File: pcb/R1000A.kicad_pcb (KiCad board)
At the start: 2 copper layers, 162 x 104 mm, 26 parts, among them J1 PCIESOCKET-X1, J10 PCIESOCKET-X1, J11 PCIESOCKET-X1, J12 PCIESOCKET-X1, J13 PCIESOCKET-X1, J14 PCIESOCKET-X1, J15 SOCKET420P-02X04-CPU, J16 SOCKET508P-01X04, J17 CONN500P-01X04, J2 PCIESOCKET-X1, J3 PCIESOCKET-X1, J4 PCIESOCKET-X1, J5 PCIESOCKET-X1, J6 PCIESOCKET-X1, J7 PCIESOCKET-X1, J8 PCIESOCKET-X1, J9 PCIESOCKET-X1, U1 LPC1769FBD100,551, U2 AP3418

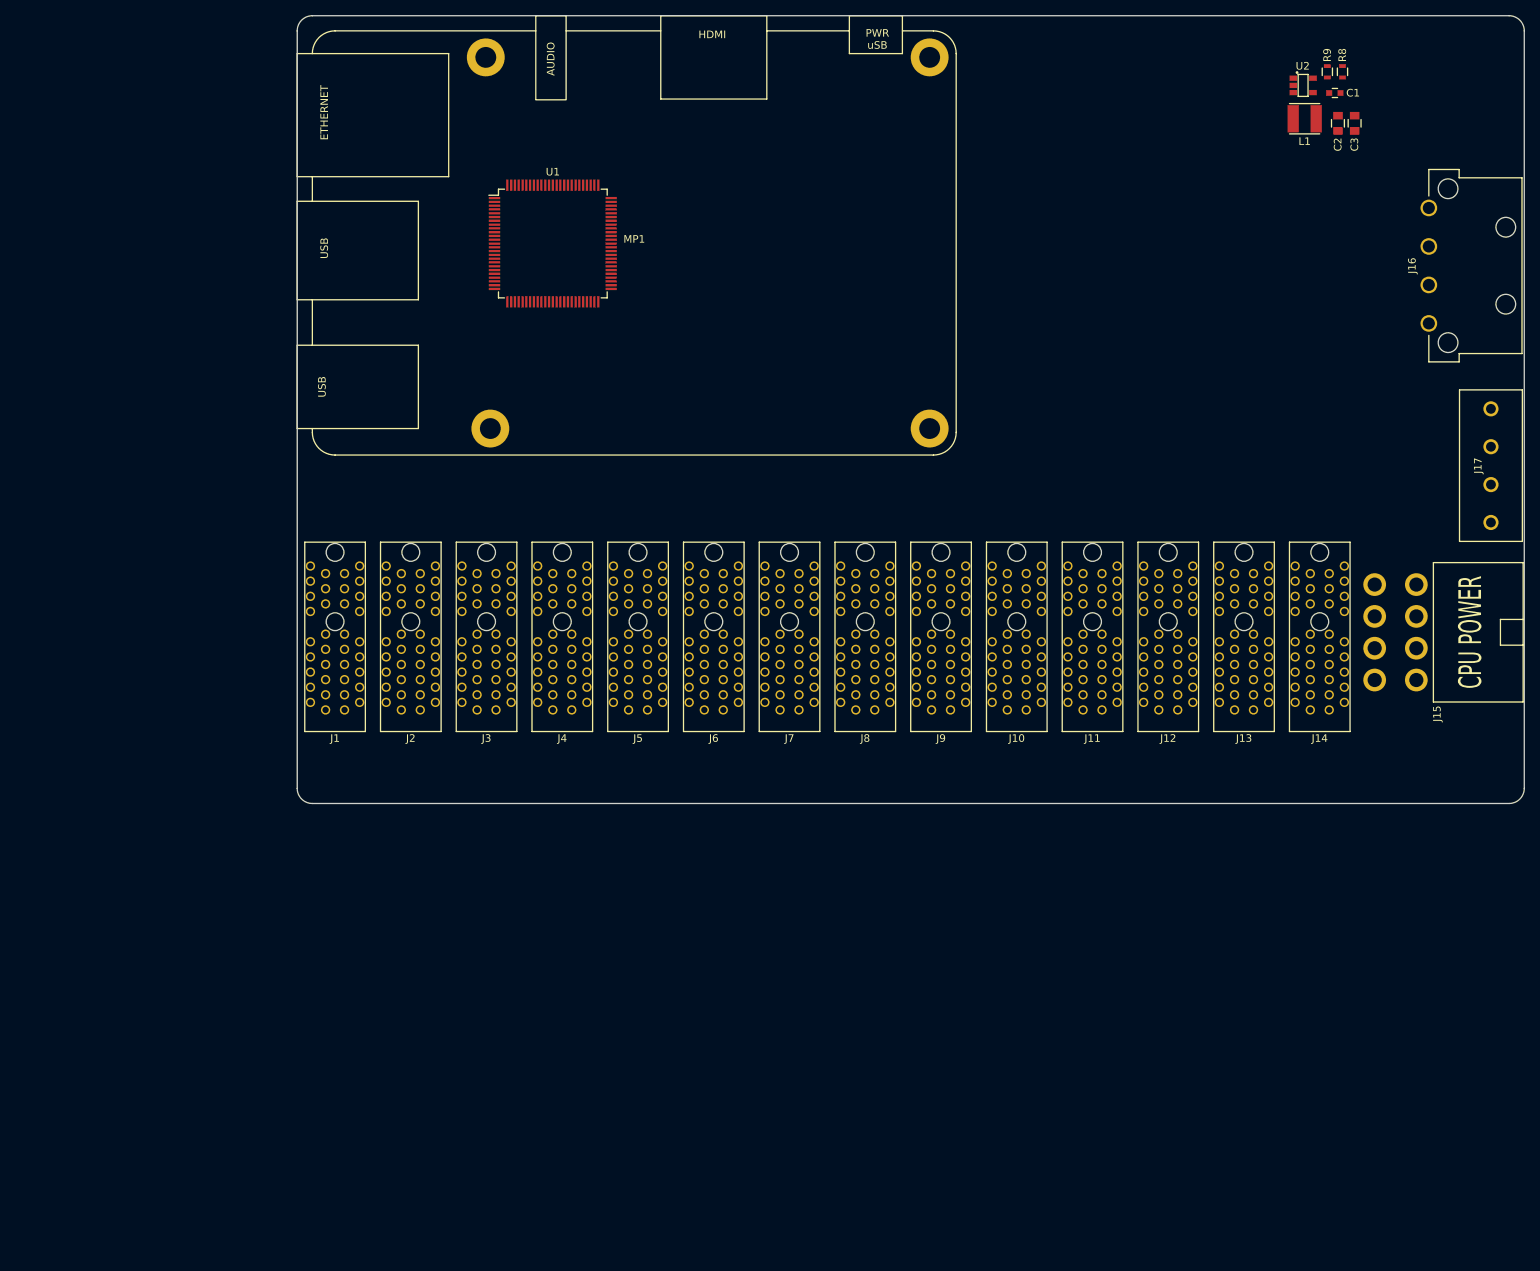
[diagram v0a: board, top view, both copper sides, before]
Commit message: wip, 90% sch complete
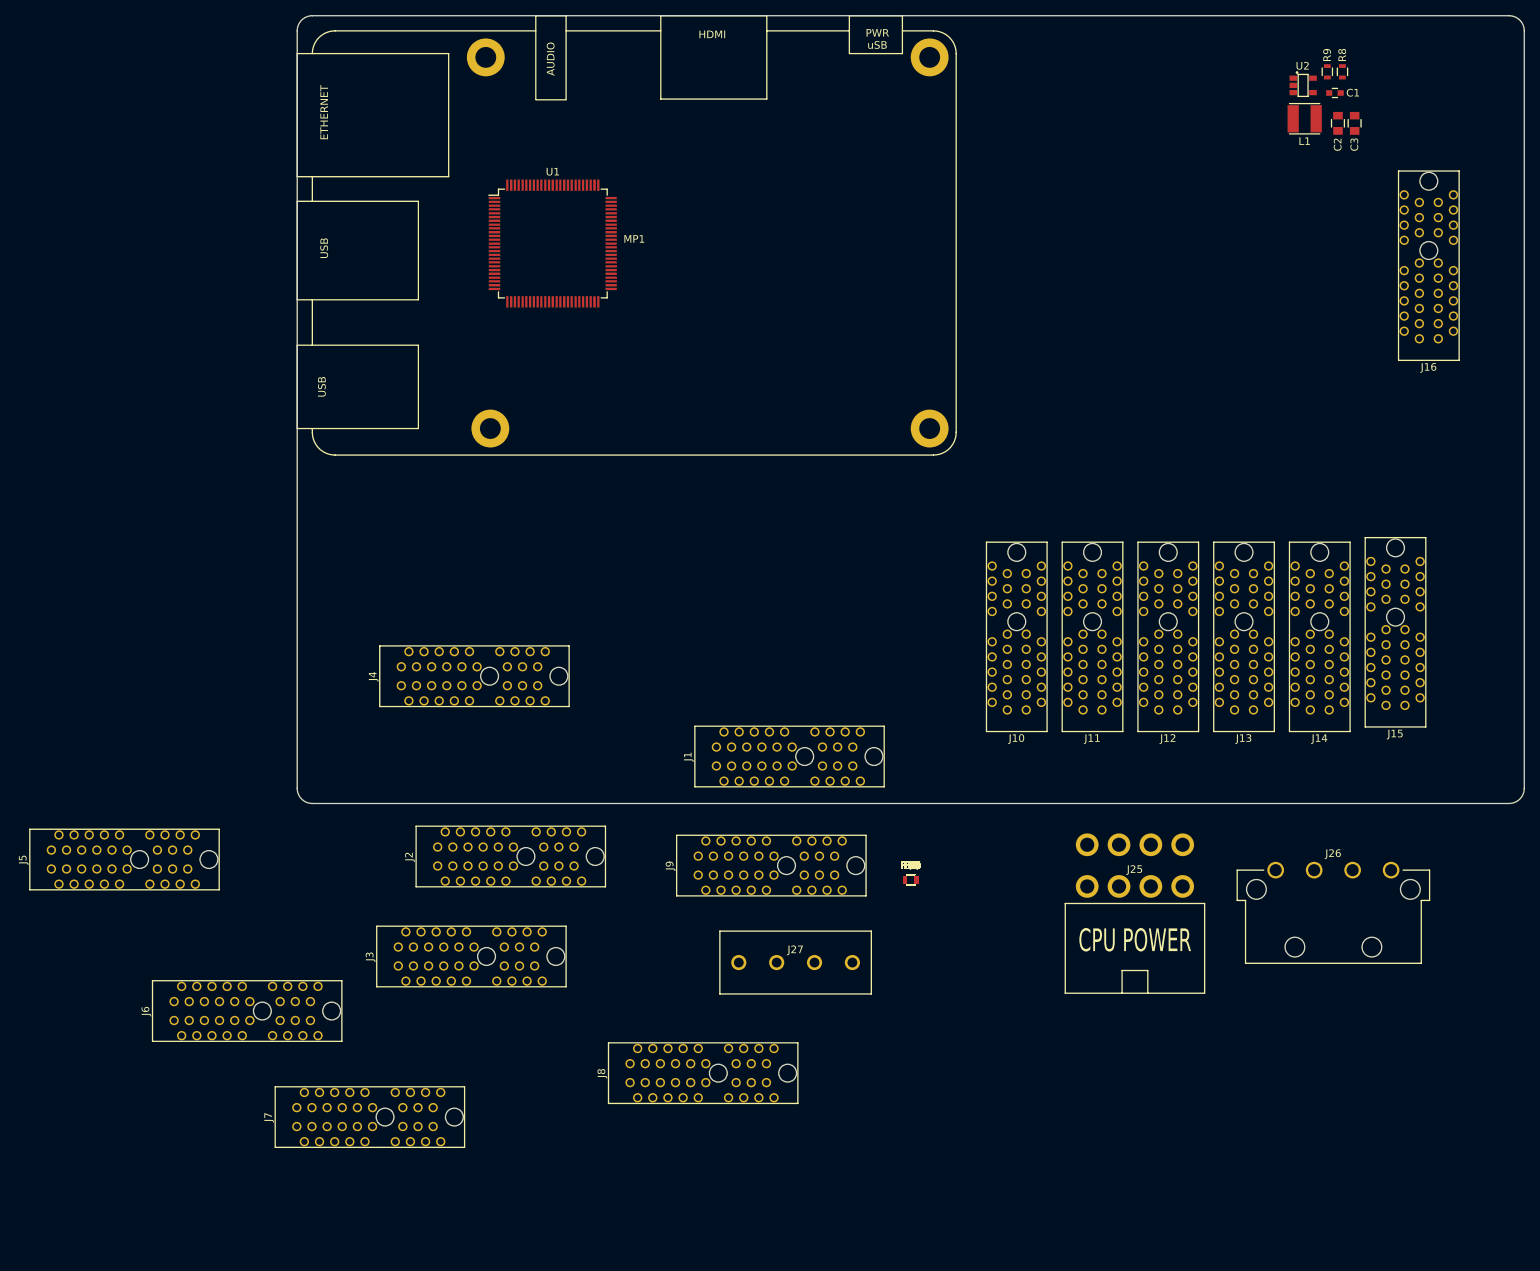
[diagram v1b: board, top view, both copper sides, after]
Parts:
- removed J17: CONN500P-01X04, Main:CONN500P-01X04
- added J25: SOCKET420P-02X04-CPU, Main:SOCKET420P-02X04, F.Cu at (175.6, 150.2)
- added J26: SOCKET508P-01X04, Main:SOCKET508P-01X04, F.Cu at (201.8, 150.8)
- added J27: CONN500P-01X04, Main:CONN500P-01X04, F.Cu at (130.8, 163.0)
- added R1, R10, R11, R12, R13, R14, R15, R16, R17, R18, R19, R2, R20, R21, R22, R23, R24, R25, R26, R27, R28, R29, R3, R30, R31, R32, R33, R34, R35, R36, R37, R38, R39, R4, R40, R41, R42, R43, R44, R45, R46, R47, R48, R49, R5, R50, R51, R52, R53, R54, R55, R56, R57, R58, R59, R6, R60, R61, R62, R63, R64, R65, R66, R7: 10k, Resistors_SMD:R_0603, F.Cu at (146.0, 152.1)
- J15: value SOCKET420P-02X04-CPU -> PCIESOCKET-X1; footprint Main:SOCKET420P-02X04 -> Main:PCIESOCKET-X1
- J16: value SOCKET508P-01X04 -> PCIESOCKET-X1; footprint Main:SOCKET508P-01X04 -> Main:PCIESOCKET-X1
- moved J7 84.2 mm to (74.6, 183.4), turned to 0 degrees
- moved J6 79.0 mm to (58.4, 169.4), turned to 0 degrees
- moved J5 73.9 mm to (42.2, 149.4), turned to 0 degrees
- moved J1 62.0 mm to (130.0, 135.8), turned to 0 degrees
- moved J8 61.4 mm to (118.6, 177.6), turned to 0 degrees
- moved J3 42.2 mm to (88.0, 162.2), turned to 0 degrees
- moved J9 37.6 mm to (127.6, 150.2), turned to 0 degrees
- moved J2 31.9 mm to (93.2, 149.0), turned to 0 degrees
- moved J4 12.7 mm to (88.4, 125.2), turned to 0 degrees
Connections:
- J1 pad A1: (no net) -> HT
- J1 pad A10: (no net) -> +5V
- J1 pad A11: (no net) -> +5V
- J1 pad A12: (no net) -> J01.PX1.A12
- J1 pad A13: (no net) -> J01.PX2.A13
- J1 pad A14: (no net) -> J01.PX3.A14
- J1 pad A15: (no net) -> J01.PX4.A15
- J1 pad A16: (no net) -> SCL0
- J1 pad A17: (no net) -> SDA0
- J1 pad A18: (no net) -> ~MRESET
- J1 pad A2: (no net) -> HT
- J1 pad A3: (no net) -> HT
- J1 pad A4: (no net) -> HT
- J1 pad A5: (no net) -> HT
- J1 pad A6: (no net) -> HT
- J1 pad A7: (no net) -> HT
- J1 pad A8: (no net) -> HT
- J1 pad A9: (no net) -> +5V
- J1 pad B1: (no net) -> GND
- J1 pad B10: (no net) -> +3V3
- J1 pad B11: (no net) -> +3V3
- J1 pad B12: (no net) -> Net-(J1-PadB12)
- J1 pad B13: (no net) -> Net-(J1-PadB13)
- J1 pad B14: (no net) -> Net-(J1-PadB14)
- J1 pad B15: (no net) -> Net-(J1-PadB15)
- J1 pad B2: (no net) -> GND
- J1 pad B3: (no net) -> GND
- J1 pad B4: (no net) -> GND
- J1 pad B5: (no net) -> GND
- J1 pad B6: (no net) -> GND
- J1 pad B7: (no net) -> GND
- J1 pad B8: (no net) -> GND
- J1 pad B9: (no net) -> +3V3
- J10 pad A1: (no net) -> HT
- J10 pad A10: (no net) -> +5V
- J10 pad A11: (no net) -> +5V
- J10 pad A12: (no net) -> J10.PX1.A12
- J10 pad A13: (no net) -> J10.PX2.A13
- J10 pad A14: (no net) -> J10.PX3.A14
- J10 pad A15: (no net) -> J10.PX4.A15
- J10 pad A16: (no net) -> SCL0
- J10 pad A17: (no net) -> SDA0
- J10 pad A18: (no net) -> ~MRESET
- J10 pad A2: (no net) -> HT
- J10 pad A3: (no net) -> HT
- J10 pad A4: (no net) -> HT
- J10 pad A5: (no net) -> HT
- J10 pad A6: (no net) -> HT
- J10 pad A7: (no net) -> HT
- J10 pad A8: (no net) -> HT
- J10 pad A9: (no net) -> +5V
- J10 pad B1: (no net) -> GND
- J10 pad B10: (no net) -> +3V3
- J10 pad B11: (no net) -> +3V3
- J10 pad B12: (no net) -> Net-(J10-PadB12)
- J10 pad B13: (no net) -> Net-(J10-PadB13)
- J10 pad B14: (no net) -> Net-(J10-PadB14)
- J10 pad B15: (no net) -> Net-(J10-PadB15)
- J10 pad B2: (no net) -> GND
- J10 pad B3: (no net) -> GND
- J10 pad B4: (no net) -> GND
- J10 pad B5: (no net) -> GND
- J10 pad B6: (no net) -> GND
- J10 pad B7: (no net) -> GND
- J10 pad B8: (no net) -> GND
- J10 pad B9: (no net) -> +3V3
- J11 pad A1: (no net) -> HT
- J11 pad A10: (no net) -> +5V
- J11 pad A11: (no net) -> +5V
- J11 pad A12: (no net) -> J11.PX1.A12
- J11 pad A13: (no net) -> J11.PX2.A13
- J11 pad A14: (no net) -> J11.PX3.A14
- J11 pad A15: (no net) -> J11.PX4.A15
- J11 pad A16: (no net) -> SCL0
- J11 pad A17: (no net) -> SDA0
- J11 pad A18: (no net) -> ~MRESET
- J11 pad A2: (no net) -> HT
- J11 pad A3: (no net) -> HT
- J11 pad A4: (no net) -> HT
- J11 pad A5: (no net) -> HT
- J11 pad A6: (no net) -> HT
- J11 pad A7: (no net) -> HT
- J11 pad A8: (no net) -> HT
- J11 pad A9: (no net) -> +5V
- J11 pad B1: (no net) -> GND
- J11 pad B10: (no net) -> +3V3
- J11 pad B11: (no net) -> +3V3
- J11 pad B12: (no net) -> Net-(J11-PadB12)
- J11 pad B13: (no net) -> Net-(J11-PadB13)
- J11 pad B14: (no net) -> Net-(J11-PadB14)
- J11 pad B15: (no net) -> Net-(J11-PadB15)
- J11 pad B2: (no net) -> GND
- J11 pad B3: (no net) -> GND
- J11 pad B4: (no net) -> GND
- J11 pad B5: (no net) -> GND
- J11 pad B6: (no net) -> GND
- J11 pad B7: (no net) -> GND
- J11 pad B8: (no net) -> GND
- J11 pad B9: (no net) -> +3V3
- J12 pad A1: (no net) -> HT
- J12 pad A10: (no net) -> +5V
- J12 pad A11: (no net) -> +5V
- J12 pad A12: (no net) -> J12.PX1.A12
- J12 pad A13: (no net) -> J12.PX2.A13
- J12 pad A14: (no net) -> J12.PX3.A14
- J12 pad A15: (no net) -> J12.PX4.A15
- J12 pad A16: (no net) -> SCL0
- J12 pad A17: (no net) -> SDA0
- J12 pad A18: (no net) -> ~MRESET
- J12 pad A2: (no net) -> HT
- J12 pad A3: (no net) -> HT
- J12 pad A4: (no net) -> HT
- J12 pad A5: (no net) -> HT
- J12 pad A6: (no net) -> HT
- J12 pad A7: (no net) -> HT
- J12 pad A8: (no net) -> HT
- J12 pad A9: (no net) -> +5V
- J12 pad B1: (no net) -> GND
- J12 pad B10: (no net) -> +3V3
- J12 pad B11: (no net) -> +3V3
- J12 pad B12: (no net) -> Net-(J12-PadB12)
- J12 pad B13: (no net) -> Net-(J12-PadB13)
- J12 pad B14: (no net) -> Net-(J12-PadB14)
- J12 pad B15: (no net) -> Net-(J12-PadB15)
- J12 pad B2: (no net) -> GND
- J12 pad B3: (no net) -> GND
- J12 pad B4: (no net) -> GND
- J12 pad B5: (no net) -> GND
- J12 pad B6: (no net) -> GND
- J12 pad B7: (no net) -> GND
- J12 pad B8: (no net) -> GND
- J12 pad B9: (no net) -> +3V3
- J13 pad A1: (no net) -> HT
- J13 pad A10: (no net) -> +5V
- J13 pad A11: (no net) -> +5V
- J13 pad A12: (no net) -> J13.PX1.A12
- J13 pad A13: (no net) -> J13.PX2.A13
- J13 pad A14: (no net) -> J13.PX3.A14
- J13 pad A15: (no net) -> J13.PX4.A15
- J13 pad A16: (no net) -> SCL0
- J13 pad A17: (no net) -> SDA0
- J13 pad A18: (no net) -> ~MRESET
- J13 pad A2: (no net) -> HT
- J13 pad A3: (no net) -> HT
- J13 pad A4: (no net) -> HT
- J13 pad A5: (no net) -> HT
- J13 pad A6: (no net) -> HT
- J13 pad A7: (no net) -> HT
- J13 pad A8: (no net) -> HT
- J13 pad A9: (no net) -> +5V
- J13 pad B1: (no net) -> GND
- J13 pad B10: (no net) -> +3V3
- J13 pad B11: (no net) -> +3V3
- J13 pad B12: (no net) -> Net-(J13-PadB12)
- J13 pad B13: (no net) -> Net-(J13-PadB13)
- J13 pad B14: (no net) -> Net-(J13-PadB14)
- J13 pad B15: (no net) -> Net-(J13-PadB15)
- J13 pad B2: (no net) -> GND
- J13 pad B3: (no net) -> GND
- J13 pad B4: (no net) -> GND
- J13 pad B5: (no net) -> GND
- J13 pad B6: (no net) -> GND
- J13 pad B7: (no net) -> GND
- J13 pad B8: (no net) -> GND
- J13 pad B9: (no net) -> +3V3
- J14 pad A1: (no net) -> HT
- J14 pad A10: (no net) -> +5V
- J14 pad A11: (no net) -> +5V
- J14 pad A12: (no net) -> J14.PX1.A12
- J14 pad A13: (no net) -> J14.PX2.A13
- J14 pad A14: (no net) -> J14.PX3.A14
- J14 pad A15: (no net) -> J14.PX4.A15
- J14 pad A16: (no net) -> SCL0
- J14 pad A17: (no net) -> SDA0
- J14 pad A18: (no net) -> ~MRESET
- J14 pad A2: (no net) -> HT
- J14 pad A3: (no net) -> HT
- J14 pad A4: (no net) -> HT
- J14 pad A5: (no net) -> HT
- J14 pad A6: (no net) -> HT
- J14 pad A7: (no net) -> HT
- J14 pad A8: (no net) -> HT
- J14 pad A9: (no net) -> +5V
- J14 pad B1: (no net) -> GND
- J14 pad B10: (no net) -> +3V3
- J14 pad B11: (no net) -> +3V3
- J14 pad B12: (no net) -> Net-(J14-PadB12)
- J14 pad B13: (no net) -> Net-(J14-PadB13)
- J14 pad B14: (no net) -> Net-(J14-PadB14)
- J14 pad B15: (no net) -> Net-(J14-PadB15)
- J14 pad B2: (no net) -> GND
- J14 pad B3: (no net) -> GND
- J14 pad B4: (no net) -> GND
- J14 pad B5: (no net) -> GND
- J14 pad B6: (no net) -> GND
- J14 pad B7: (no net) -> GND
- J14 pad B8: (no net) -> GND
- J14 pad B9: (no net) -> +3V3
- J2 pad A1: (no net) -> HT
- J2 pad A10: (no net) -> +5V
- J2 pad A11: (no net) -> +5V
- J2 pad A12: (no net) -> J02.PX1.A12
- J2 pad A13: (no net) -> J02.PX2.A13
- J2 pad A14: (no net) -> J02.PX3.A14
- J2 pad A15: (no net) -> J02.PX4.A15
- J2 pad A16: (no net) -> SCL0
- J2 pad A17: (no net) -> SDA0
- J2 pad A18: (no net) -> ~MRESET
- J2 pad A2: (no net) -> HT
- J2 pad A3: (no net) -> HT
- J2 pad A4: (no net) -> HT
- J2 pad A5: (no net) -> HT
- J2 pad A6: (no net) -> HT
- J2 pad A7: (no net) -> HT
- J2 pad A8: (no net) -> HT
- J2 pad A9: (no net) -> +5V
- J2 pad B1: (no net) -> GND
- J2 pad B10: (no net) -> +3V3
- J2 pad B11: (no net) -> +3V3
- J2 pad B12: (no net) -> Net-(J2-PadB12)
- J2 pad B13: (no net) -> Net-(J2-PadB13)
- J2 pad B14: (no net) -> Net-(J2-PadB14)
- J2 pad B15: (no net) -> Net-(J2-PadB15)
- J2 pad B2: (no net) -> GND
- J2 pad B3: (no net) -> GND
- J2 pad B4: (no net) -> GND
- J2 pad B5: (no net) -> GND
- J2 pad B6: (no net) -> GND
- J2 pad B7: (no net) -> GND
- J2 pad B8: (no net) -> GND
- J2 pad B9: (no net) -> +3V3
- J3 pad A1: (no net) -> HT
- J3 pad A10: (no net) -> Net-(J3-PadA10)
- J3 pad A11: (no net) -> Net-(J3-PadA10)
- J3 pad A12: (no net) -> J03.PX1.A12
- J3 pad A13: (no net) -> J03.PX2.A13
- J3 pad A14: (no net) -> J03.PX3.A14
- J3 pad A15: (no net) -> J03.PX4.A15
- J3 pad A16: (no net) -> SCL0
- J3 pad A17: (no net) -> SDA0
- J3 pad A18: (no net) -> ~MRESET
- J3 pad A2: (no net) -> HT
- J3 pad A3: (no net) -> HT
- J3 pad A4: (no net) -> HT
- J3 pad A5: (no net) -> HT
- J3 pad A6: (no net) -> HT
- J3 pad A7: (no net) -> HT
- J3 pad A8: (no net) -> HT
- J3 pad A9: (no net) -> Net-(J3-PadA10)
- J3 pad B1: (no net) -> GND
- J3 pad B10: (no net) -> +3V3
- J3 pad B11: (no net) -> +3V3
- J3 pad B12: (no net) -> Net-(J3-PadB12)
- J3 pad B13: (no net) -> Net-(J3-PadB13)
- J3 pad B14: (no net) -> Net-(J3-PadB14)
- J3 pad B15: (no net) -> Net-(J3-PadB15)
- J3 pad B2: (no net) -> GND
- J3 pad B3: (no net) -> GND
- J3 pad B4: (no net) -> GND
- J3 pad B5: (no net) -> GND
- J3 pad B6: (no net) -> GND
- J3 pad B7: (no net) -> GND
- J3 pad B8: (no net) -> GND
- J3 pad B9: (no net) -> +3V3
- J4 pad A1: (no net) -> HT
- J4 pad A10: (no net) -> +5V
- J4 pad A11: (no net) -> +5V
- J4 pad A12: (no net) -> J04.PX1.A12
- J4 pad A13: (no net) -> J04.PX2.A13
- J4 pad A14: (no net) -> J04.PX3.A14
- J4 pad A15: (no net) -> J04.PX4.A15
- J4 pad A16: (no net) -> SCL0
- J4 pad A17: (no net) -> SDA0
- J4 pad A18: (no net) -> ~MRESET
- J4 pad A2: (no net) -> HT
- J4 pad A3: (no net) -> HT
- J4 pad A4: (no net) -> HT
- J4 pad A5: (no net) -> HT
- J4 pad A6: (no net) -> HT
- J4 pad A7: (no net) -> HT
- J4 pad A8: (no net) -> HT
- J4 pad A9: (no net) -> +5V
- J4 pad B1: (no net) -> GND
- J4 pad B10: (no net) -> +3V3
- J4 pad B11: (no net) -> +3V3
- J4 pad B12: (no net) -> Net-(J4-PadB12)
- J4 pad B13: (no net) -> Net-(J4-PadB13)
- J4 pad B14: (no net) -> Net-(J4-PadB14)
- J4 pad B15: (no net) -> Net-(J4-PadB15)
- J4 pad B2: (no net) -> GND
- J4 pad B3: (no net) -> GND
- J4 pad B4: (no net) -> GND
- J4 pad B5: (no net) -> GND
- J4 pad B6: (no net) -> GND
- J4 pad B7: (no net) -> GND
- J4 pad B8: (no net) -> GND
- J4 pad B9: (no net) -> +3V3
- J5 pad A1: (no net) -> HT
- J5 pad A10: (no net) -> +5V
- J5 pad A11: (no net) -> +5V
- J5 pad A12: (no net) -> J05.PX1.A12
- J5 pad A13: (no net) -> J05.PX2.A13
- J5 pad A14: (no net) -> J05.PX3.A14
- J5 pad A15: (no net) -> J05.PX4.A15
- J5 pad A16: (no net) -> SCL0
- J5 pad A17: (no net) -> SDA0
- J5 pad A18: (no net) -> ~MRESET
- J5 pad A2: (no net) -> HT
- J5 pad A3: (no net) -> HT
- J5 pad A4: (no net) -> HT
- J5 pad A5: (no net) -> HT
- J5 pad A6: (no net) -> HT
- J5 pad A7: (no net) -> HT
- J5 pad A8: (no net) -> HT
- J5 pad A9: (no net) -> +5V
- J5 pad B1: (no net) -> GND
- J5 pad B10: (no net) -> +3V3
- J5 pad B11: (no net) -> +3V3
- J5 pad B12: (no net) -> Net-(J5-PadB12)
- J5 pad B13: (no net) -> Net-(J5-PadB13)
- J5 pad B14: (no net) -> Net-(J5-PadB14)
- J5 pad B15: (no net) -> Net-(J5-PadB15)
- J5 pad B2: (no net) -> GND
- J5 pad B3: (no net) -> GND
- J5 pad B4: (no net) -> GND
- J5 pad B5: (no net) -> GND
- J5 pad B6: (no net) -> GND
- J5 pad B7: (no net) -> GND
- J5 pad B8: (no net) -> GND
- J5 pad B9: (no net) -> +3V3
- J6 pad A1: (no net) -> HT
- J6 pad A10: (no net) -> +5V
- J6 pad A11: (no net) -> +5V
- J6 pad A12: (no net) -> J06.PX1.A12
- J6 pad A13: (no net) -> J06.PX2.A13
- J6 pad A14: (no net) -> J06.PX3.A14
- J6 pad A15: (no net) -> J06.PX4.A15
- J6 pad A16: (no net) -> SCL0
- J6 pad A17: (no net) -> SDA0
- J6 pad A18: (no net) -> ~MRESET
- J6 pad A2: (no net) -> HT
- J6 pad A3: (no net) -> HT
- J6 pad A4: (no net) -> HT
- J6 pad A5: (no net) -> HT
- J6 pad A6: (no net) -> HT
- J6 pad A7: (no net) -> HT
- J6 pad A8: (no net) -> HT
- J6 pad A9: (no net) -> +5V
- J6 pad B1: (no net) -> GND
- J6 pad B10: (no net) -> +3V3
- J6 pad B11: (no net) -> +3V3
- J6 pad B12: (no net) -> Net-(J6-PadB12)
- J6 pad B13: (no net) -> Net-(J6-PadB13)
- J6 pad B14: (no net) -> Net-(J6-PadB14)
- J6 pad B15: (no net) -> Net-(J6-PadB15)
- J6 pad B2: (no net) -> GND
- J6 pad B3: (no net) -> GND
- J6 pad B4: (no net) -> GND
- J6 pad B5: (no net) -> GND
- J6 pad B6: (no net) -> GND
- J6 pad B7: (no net) -> GND
- J6 pad B8: (no net) -> GND
- J6 pad B9: (no net) -> +3V3
- J7 pad A1: (no net) -> HT
- J7 pad A10: (no net) -> +5V
- J7 pad A11: (no net) -> +5V
- J7 pad A12: (no net) -> J07.PX1.A12
- J7 pad A13: (no net) -> J07.PX2.A13
- J7 pad A14: (no net) -> J07.PX3.A14
- J7 pad A15: (no net) -> J07.PX4.A15
- J7 pad A16: (no net) -> SCL0
- J7 pad A17: (no net) -> SDA0
- J7 pad A18: (no net) -> ~MRESET
- J7 pad A2: (no net) -> HT
- J7 pad A3: (no net) -> HT
- J7 pad A4: (no net) -> HT
- J7 pad A5: (no net) -> HT
- J7 pad A6: (no net) -> HT
- J7 pad A7: (no net) -> HT
- J7 pad A8: (no net) -> HT
- J7 pad A9: (no net) -> +5V
- J7 pad B1: (no net) -> GND
- J7 pad B10: (no net) -> +3V3
- J7 pad B11: (no net) -> +3V3
- J7 pad B12: (no net) -> Net-(J7-PadB12)
- J7 pad B13: (no net) -> Net-(J7-PadB13)
- J7 pad B14: (no net) -> Net-(J7-PadB14)
- J7 pad B15: (no net) -> Net-(J7-PadB15)
- J7 pad B2: (no net) -> GND
- J7 pad B3: (no net) -> GND
- J7 pad B4: (no net) -> GND
- J7 pad B5: (no net) -> GND
- J7 pad B6: (no net) -> GND
- J7 pad B7: (no net) -> GND
- J7 pad B8: (no net) -> GND
- J7 pad B9: (no net) -> +3V3
- J8 pad A1: (no net) -> HT
- J8 pad A10: (no net) -> +5V
- J8 pad A11: (no net) -> +5V
- J8 pad A12: (no net) -> J08.PX1.A12
- J8 pad A13: (no net) -> J08.PX2.A13
- J8 pad A14: (no net) -> J08.PX3.A14
- J8 pad A15: (no net) -> J08.PX4.A15
- J8 pad A16: (no net) -> SCL0
- J8 pad A17: (no net) -> SDA0
- J8 pad A18: (no net) -> ~MRESET
- J8 pad A2: (no net) -> HT
- J8 pad A3: (no net) -> HT
- J8 pad A4: (no net) -> HT
- J8 pad A5: (no net) -> HT
- J8 pad A6: (no net) -> HT
- J8 pad A7: (no net) -> HT
- J8 pad A8: (no net) -> HT
- J8 pad A9: (no net) -> +5V
- J8 pad B1: (no net) -> GND
- J8 pad B10: (no net) -> +3V3
- J8 pad B11: (no net) -> +3V3
- J8 pad B12: (no net) -> Net-(J8-PadB12)
- J8 pad B13: (no net) -> Net-(J8-PadB13)
- J8 pad B14: (no net) -> Net-(J8-PadB14)
- J8 pad B15: (no net) -> Net-(J8-PadB15)
- J8 pad B2: (no net) -> GND
- J8 pad B3: (no net) -> GND
- J8 pad B4: (no net) -> GND
- J8 pad B5: (no net) -> GND
- J8 pad B6: (no net) -> GND
- J8 pad B7: (no net) -> GND
- J8 pad B8: (no net) -> GND
- J8 pad B9: (no net) -> +3V3
- J9 pad A1: (no net) -> HT
- J9 pad A10: (no net) -> +5V
- J9 pad A11: (no net) -> +5V
- J9 pad A12: (no net) -> J09.PX1.A12
- J9 pad A13: (no net) -> J09.PX2.A13
- J9 pad A14: (no net) -> J09.PX3.A14
- J9 pad A15: (no net) -> J09.PX4.A15
- J9 pad A16: (no net) -> SCL0
- J9 pad A17: (no net) -> SDA0
- J9 pad A18: (no net) -> ~MRESET
- J9 pad A2: (no net) -> HT
- J9 pad A3: (no net) -> HT
- J9 pad A4: (no net) -> HT
- J9 pad A5: (no net) -> HT
- J9 pad A6: (no net) -> HT
- J9 pad A7: (no net) -> HT
- J9 pad A8: (no net) -> HT
- J9 pad A9: (no net) -> +5V
- J9 pad B1: (no net) -> GND
- J9 pad B10: (no net) -> +3V3
- J9 pad B11: (no net) -> +3V3
- J9 pad B12: (no net) -> Net-(J9-PadB12)
- J9 pad B13: (no net) -> Net-(J9-PadB13)
- J9 pad B14: (no net) -> Net-(J9-PadB14)
- J9 pad B15: (no net) -> Net-(J9-PadB15)
- J9 pad B2: (no net) -> GND
- J9 pad B3: (no net) -> GND
- J9 pad B4: (no net) -> GND
- J9 pad B5: (no net) -> GND
- J9 pad B6: (no net) -> GND
- J9 pad B7: (no net) -> GND
- J9 pad B8: (no net) -> GND
- J9 pad B9: (no net) -> +3V3
- U1 pad 20: (no net) -> J03.PX1.A12
- U1 pad 21: (no net) -> J03.PX2.A13
- U1 pad 24: (no net) -> SCL0
- U1 pad 25: (no net) -> SDA0
- U1 pad 26: (no net) -> J12.PX1.A12
- U1 pad 27: (no net) -> J12.PX2.A13
- U1 pad 32: (no net) -> J08.PX1.A12
- U1 pad 33: (no net) -> J12.PX3.A14
- U1 pad 34: (no net) -> J08.PX2.A13
- U1 pad 35: (no net) -> J12.PX4.A15
- U1 pad 36: (no net) -> J13.PX1.A12
- U1 pad 37: (no net) -> J13.PX2.A13
- U1 pad 38: (no net) -> J13.PX3.A14
- U1 pad 39: (no net) -> J13.PX4.A15
- U1 pad 40: (no net) -> J14.PX1.A12
- U1 pad 43: (no net) -> J14.PX2.A13
- U1 pad 44: (no net) -> J14.PX3.A14
- U1 pad 45: (no net) -> J14.PX4.A15
- U1 pad 46: (no net) -> J10.PX1.A12
- U1 pad 47: (no net) -> J10.PX2.A13
- U1 pad 48: (no net) -> J10.PX4.A15
- U1 pad 49: (no net) -> J10.PX3.A14
- U1 pad 50: (no net) -> J11.PX1.A12
- U1 pad 51: (no net) -> J11.PX2.A13
- U1 pad 52: (no net) -> J11.PX3.A14
- U1 pad 53: (no net) -> J11.PX4.A15
- U1 pad 56: (no net) -> J09.PX1.A12
- U1 pad 57: (no net) -> J09.PX2.A13
- U1 pad 58: (no net) -> J09.PX3.A14
- U1 pad 59: (no net) -> J09.PX4.A15
- U1 pad 6: (no net) -> J02.PX3.A14
- U1 pad 60: (no net) -> J07.PX1.A12
- U1 pad 61: (no net) -> J07.PX2.A13
- U1 pad 62: (no net) -> J07.PX4.A15
- U1 pad 63: (no net) -> J07.PX3.A14
- U1 pad 64: (no net) -> J04.PX3.A14
- U1 pad 65: (no net) -> J04.PX4.A15
- U1 pad 66: (no net) -> J04.PX1.A12
- U1 pad 67: (no net) -> J04.PX2.A13
- U1 pad 68: (no net) -> J08.PX3.A14
- U1 pad 69: (no net) -> J08.PX4.A15
- U1 pad 7: (no net) -> J02.PX4.A15
- U1 pad 70: (no net) -> J05.PX1.A12
- U1 pad 73: (no net) -> J05.PX2.A13
- U1 pad 74: (no net) -> J05.PX3.A14
- U1 pad 75: (no net) -> J05.PX4.A15
- U1 pad 76: (no net) -> J01.PX1.A12
- U1 pad 77: (no net) -> J01.PX2.A13
- U1 pad 78: (no net) -> J01.PX4.A15
- U1 pad 79: (no net) -> J01.PX3.A14
- U1 pad 8: (no net) -> J02.PX2.A13
- U1 pad 80: (no net) -> J06.PX2.A13
- U1 pad 81: (no net) -> J06.PX1.A12
- U1 pad 82: (no net) -> J06.PX4.A15
- U1 pad 85: (no net) -> J06.PX3.A14
- U1 pad 86: (no net) -> J15.PX1.A12
- U1 pad 87: (no net) -> J15.PX2.A13
- U1 pad 88: (no net) -> J15.PX3.A14
- U1 pad 89: (no net) -> J15.PX4.A15
- U1 pad 9: (no net) -> J02.PX1.A12
- U1 pad 90: (no net) -> J16.PX1.A12
- U1 pad 91: (no net) -> J16.PX2.A13
- U1 pad 92: (no net) -> J16.PX3.A14
- U1 pad 93: (no net) -> J16.PX4.A15
- U1 pad 95: (no net) -> ~MRESET
- U1 pad 98: (no net) -> J03.PX4.A15
- U1 pad 99: (no net) -> J03.PX3.A14

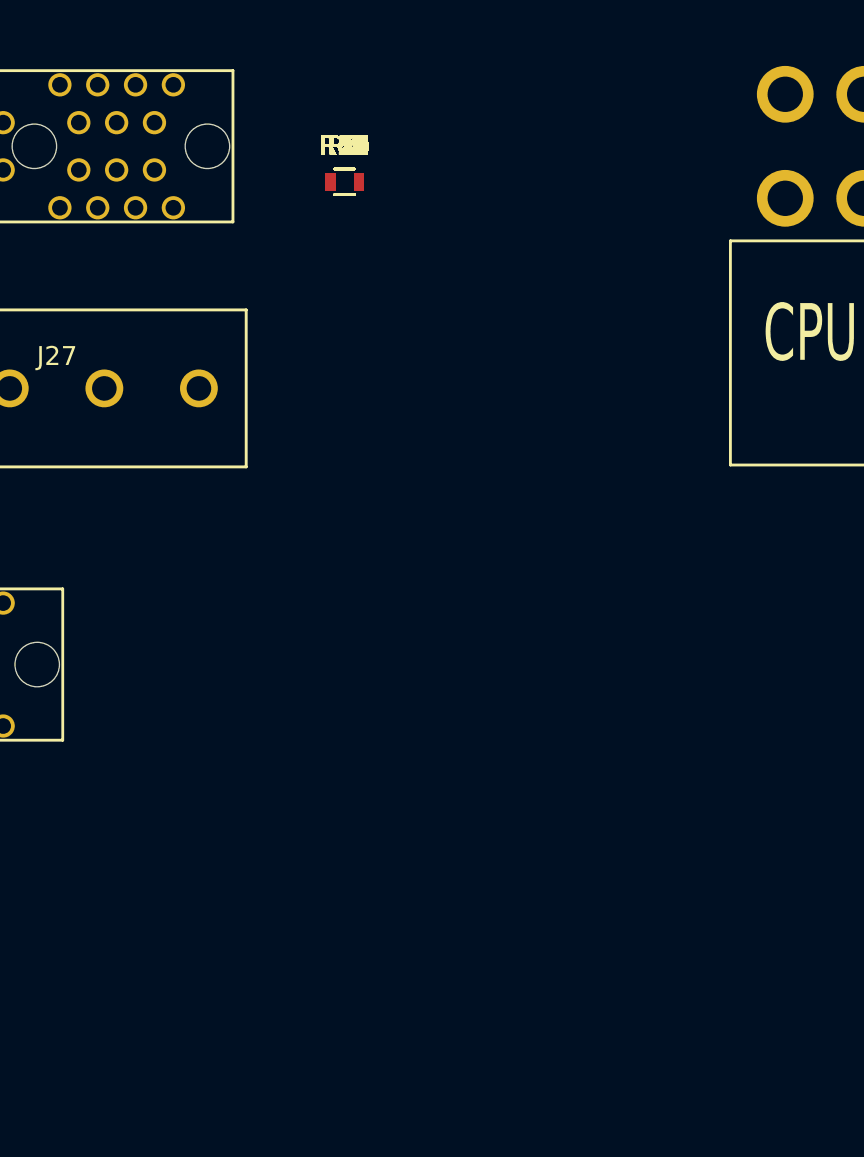
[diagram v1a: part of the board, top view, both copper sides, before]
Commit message: completed schematics
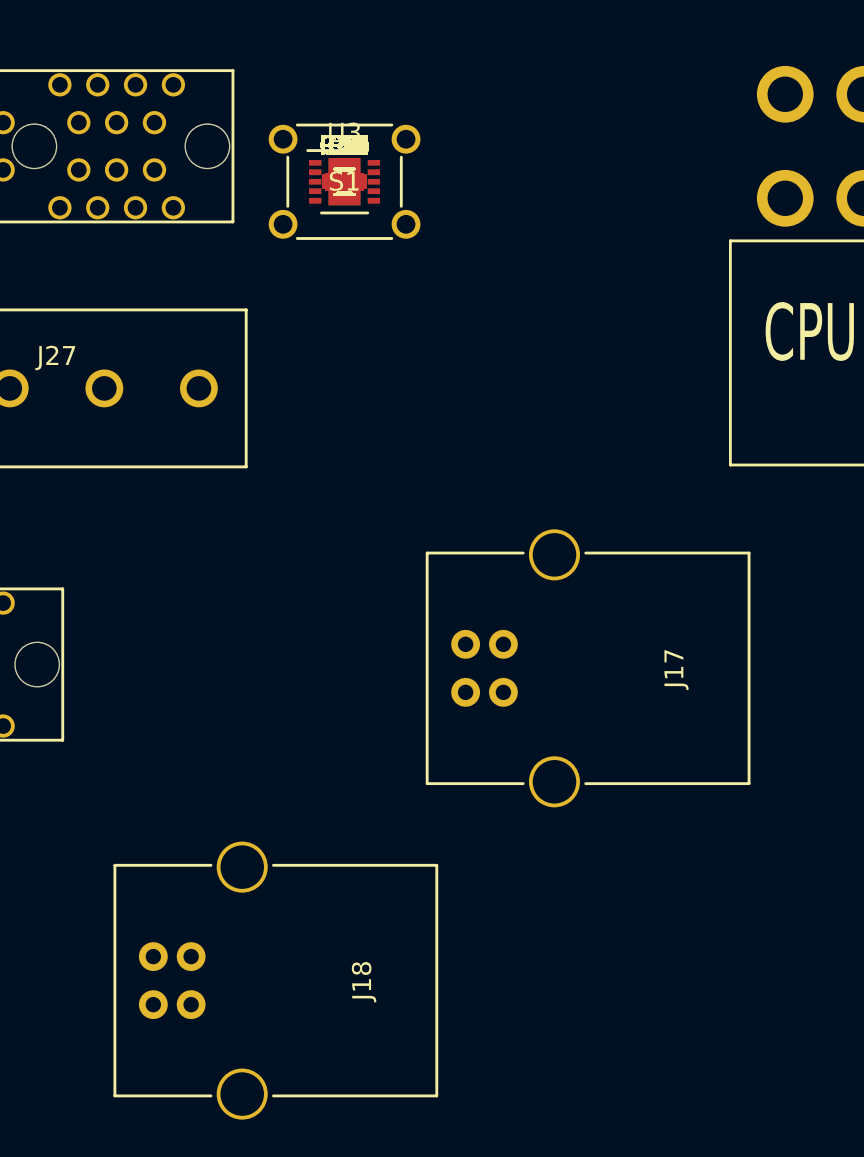
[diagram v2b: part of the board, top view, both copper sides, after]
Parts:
- added C10, C11, C12, C4, C5, C6, C7: 0.1u, Capacitors_SMD:C_0603, F.Cu at (146.0, 152.1)
- added C8, C9: 12pF, Capacitors_SMD:C_0603, F.Cu at (146.0, 152.1)
- added J17: USB_B_RECEPTACLE, Main:USB_B_RECEPTACLE, F.Cu at (152.4, 176.5)
- added J18: USB_B_RECEPTACLE, Main:USB_B_RECEPTACLE, F.Cu at (135.9, 193.0)
- added R67, R68, R69: 10k, Resistors_SMD:R_0603, F.Cu at (146.0, 152.1)
- added S1: SPST_PUSHBTN, Main:SPST_PUSHBTN, F.Cu at (146.0, 152.1)
- added U3: NX3DV221, Main:DFN50P300X300X085-10NT250X170, F.Cu at (146.0, 152.1)
- U1: footprint Main:QFP050P1400X1400X160-100 -> Main:QFP50P1400X1400X160-100
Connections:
- U1 pad 10: (no net) -> Net-(C10-Pad1)
- U1 pad 11: (no net) -> GND
- U1 pad 12: (no net) -> Net-(C10-Pad1)
- U1 pad 15: (no net) -> GND
- U1 pad 17: (no net) -> Net-(R67-Pad2)
- U1 pad 19: (no net) -> +3V3
- U1 pad 22: (no net) -> /XTAL1
- U1 pad 23: (no net) -> /XTAL2
- U1 pad 28: (no net) -> +3V3
- U1 pad 29: (no net) -> /MCU_USB_D+
- U1 pad 30: (no net) -> /MCU_USB_D-
- U1 pad 31: (no net) -> GND
- U1 pad 41: (no net) -> GND
- U1 pad 42: (no net) -> +3V3
- U1 pad 54: (no net) -> +3V3
- U1 pad 55: (no net) -> GND
- U1 pad 71: (no net) -> +3V3
- U1 pad 72: (no net) -> GND
- U1 pad 83: (no net) -> GND
- U1 pad 84: (no net) -> +3V3
- U1 pad 96: (no net) -> +3V3
- U1 pad 97: (no net) -> GND
